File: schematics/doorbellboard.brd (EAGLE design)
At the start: 25.4 x 68.6 mm, 8 parts

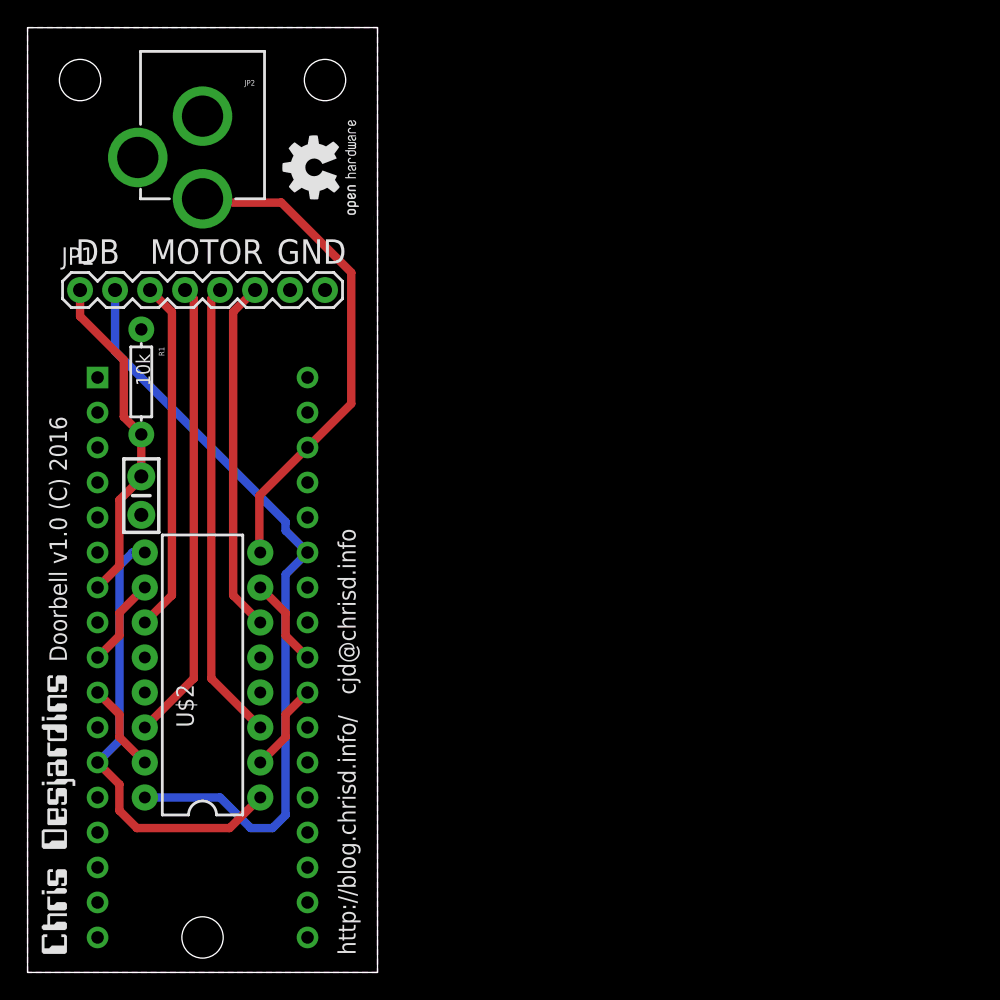
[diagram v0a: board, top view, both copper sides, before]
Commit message: Rotate board
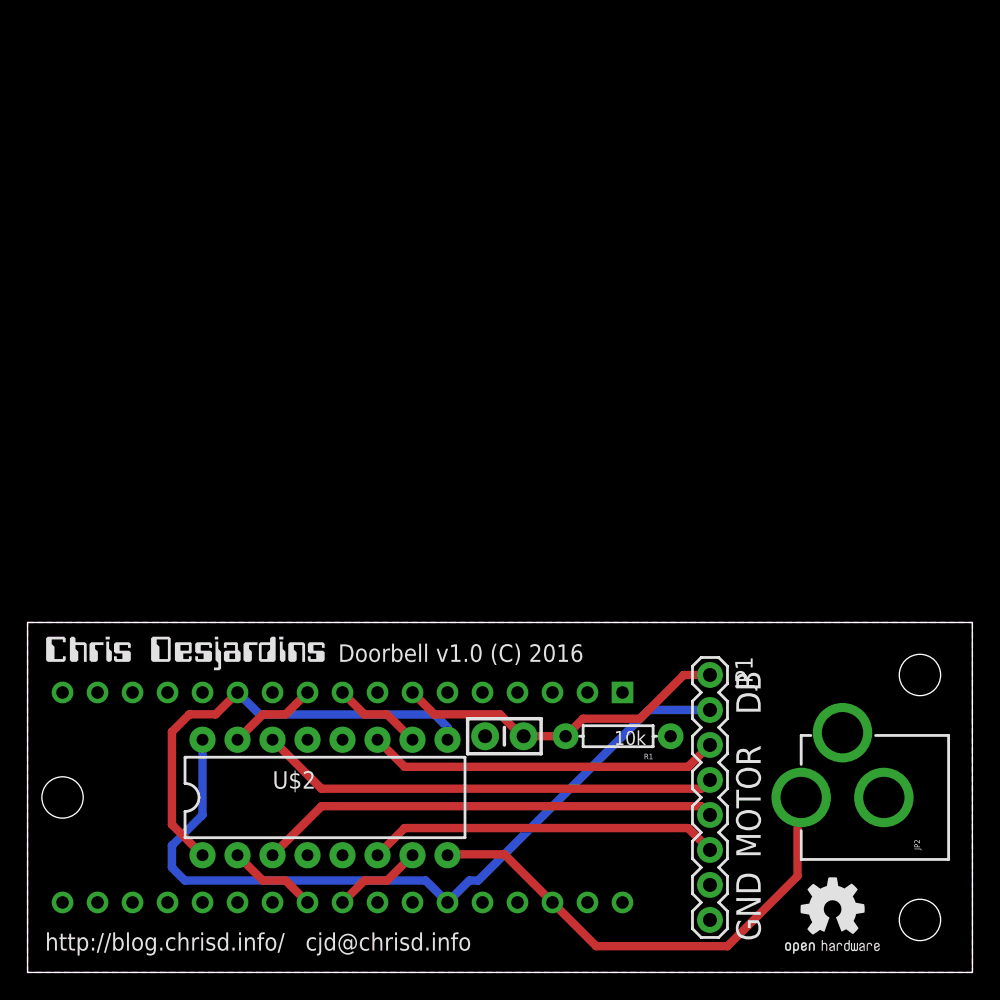
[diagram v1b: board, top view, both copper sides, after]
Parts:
- moved JP2 80.8 mm to (69.8, 12.7), turned to 90 degrees
- moved U$4 61.8 mm to (54.6, 0.32), turned to 0 degrees
- moved JP1 53.6 mm to (49.5, 21.6), turned to 270 degrees
- moved R1 43.1 mm to (42.9, 17.1), turned to 180 degrees
- moved C1 31.6 mm to (34.6, 17.1), turned to 0 degrees
- moved U$1 23.4 mm to (-1.27, 21.6), turned to 270 degrees
- moved U$3 21.3 mm to (1.27, 22.5), turned to 0 degrees
- moved U$2 12.6 mm to (21.6, 12.7), turned to 0 degrees
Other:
- board size 25.4 x 68.6 mm -> 68.6 x 25.4 mm
